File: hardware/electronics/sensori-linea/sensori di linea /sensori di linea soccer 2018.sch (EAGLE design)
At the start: 21 parts, among them T1 BP103, T2 BP103, T3 BP103, T4 BP103

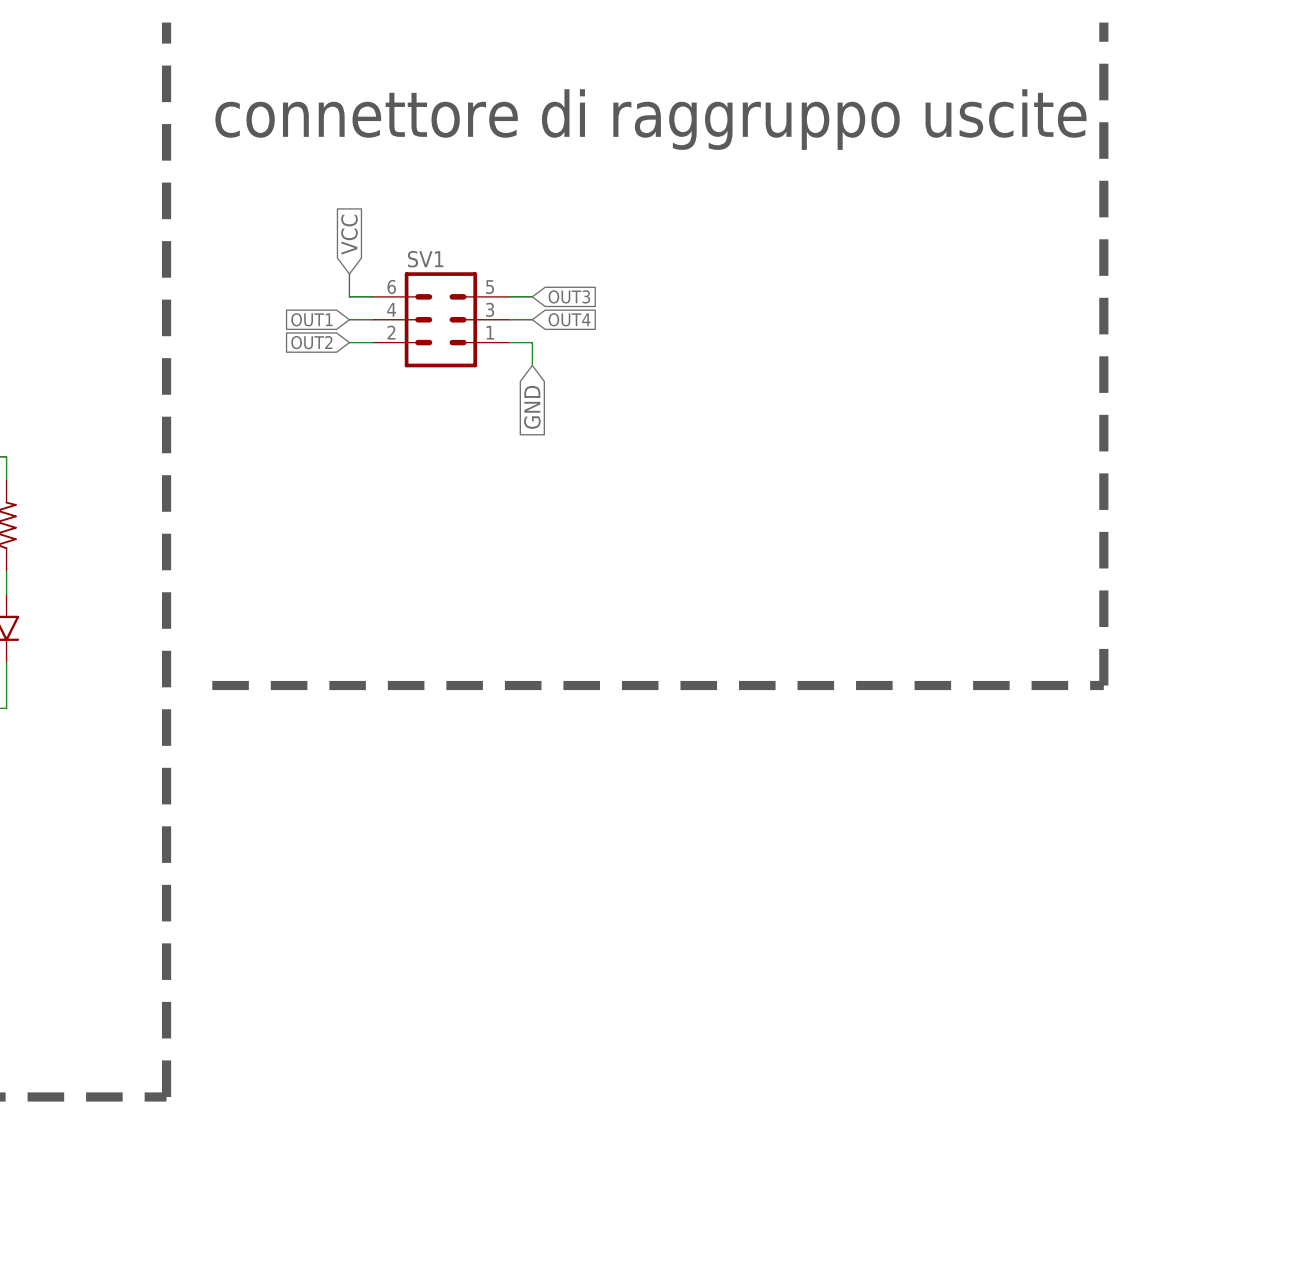
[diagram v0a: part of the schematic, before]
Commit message: aggiornamenti sensori
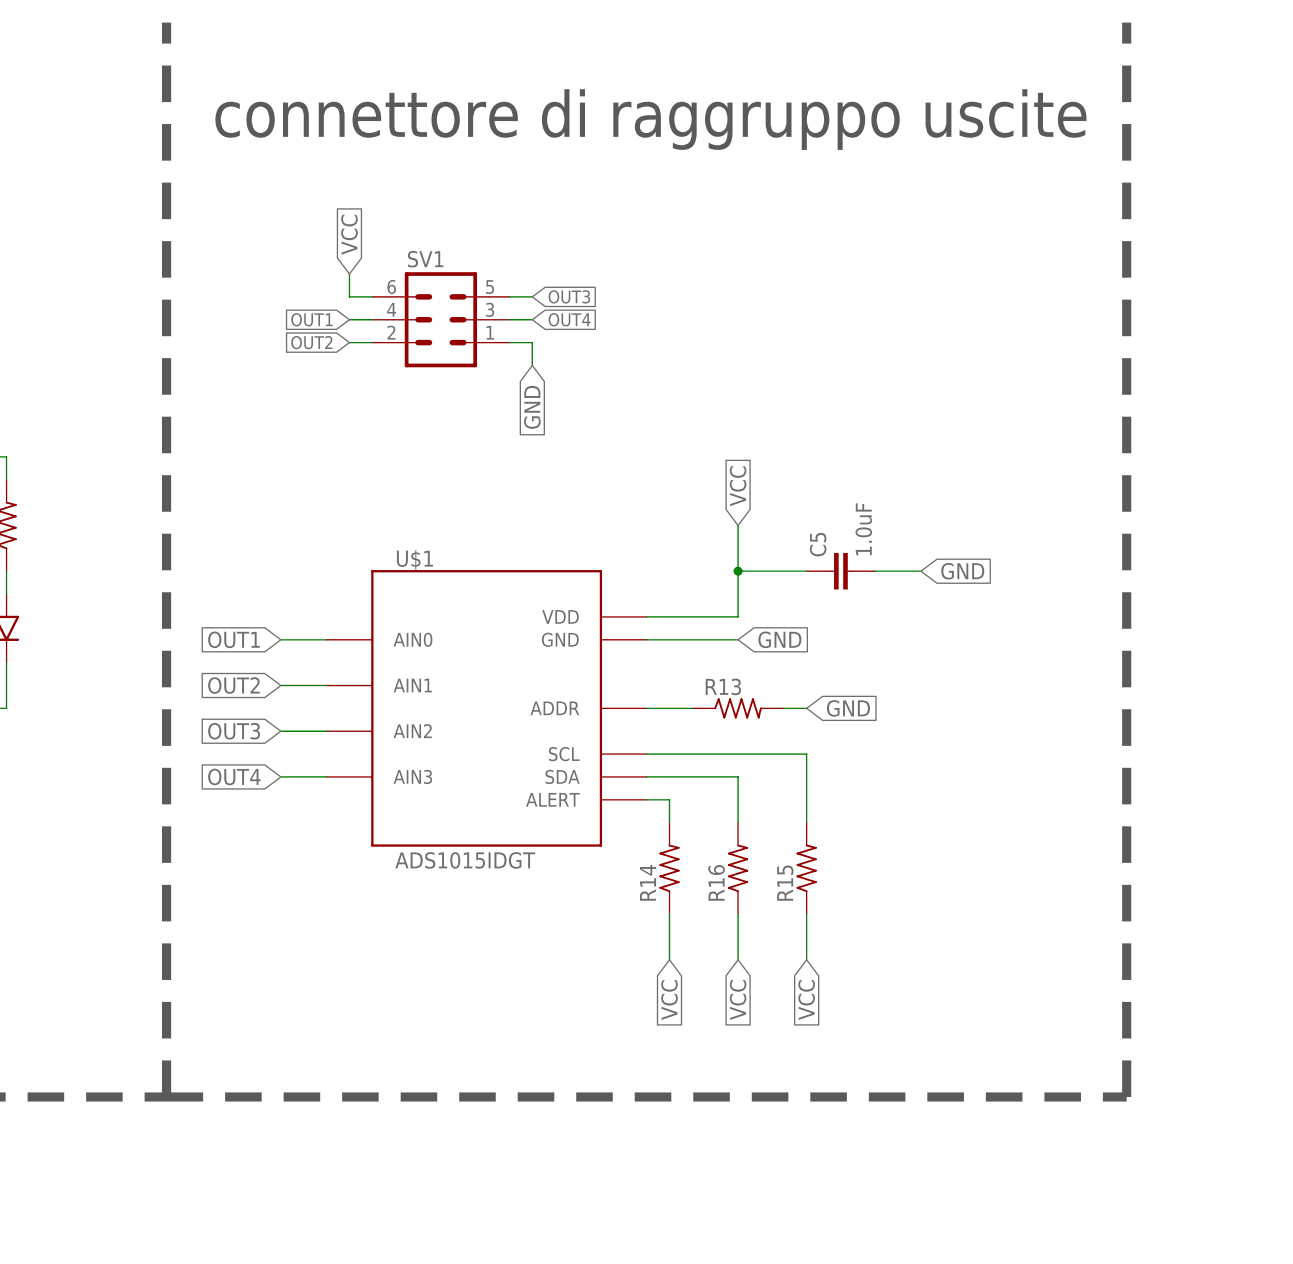
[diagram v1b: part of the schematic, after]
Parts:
- added C5: 1.0uF, SparkFun-Capacitors:1.0UF-0402-16V-10%
- added R13, R14, R15, R16: (no value), resistor:R-US_0204/7
- added U$1: ADS1015IDGT, bt_adc:ADS1015IDGT
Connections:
- new net N$1: R13.1, U$1.ADDR
- new net N$6: R16.2, U$1.SDA
- new net N$7: R14.2, U$1.ALERT
- new net N$8: R15.2, U$1.SCL
- net GND: now also C5.2, R13.2, U$1.GND
- net OUT1: now also U$1.AIN0
- net OUT2: now also U$1.AIN1
- net OUT3: now also U$1.AIN2
- net OUT4: now also U$1.AIN3
- net VCC: now also C5.1, R14.1, R15.1, R16.1, U$1.VDD
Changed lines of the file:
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@@
 <layers>
 <layer number="1" name="Top" color="4" fill="1" visible="no" active="no"/>
+<layer number="2" name="Route2" color="1" fill="3" visible="no" active="no"/>
+<layer number="3" name="Route3" color="4" fill="3" visible="no" active="no"/>
+<layer number="4" name="Route4" color="1" fill="4" visible="no" active="no"/>
+<layer number="5" name="Route5" color="4" fill="4" visible="no" active="no"/>
+<layer number="6" name="Route6" color="1" fill="8" visible="no" active="no"/>
+<layer number="7" name="Route7" color="4" fill="8" visible="no" active="no"/>
+<layer number="8" name="Route8" color="1" fill="2" visible="no" active="no"/>
+<layer number="9" name="Route9" color="4" fill="2" visible="no" active="no"/>
+<layer number="10" name="Route10" color="1" fill="7" visible="no" active="no"/>
+<layer number="11" name="Route11" color="4" fill="7" visible="no" active="no"/>
+<layer number="12" name="Route12" color="1" fill="5" visible="no" active="no"/>
+<layer number="13" name="Route13" color="4" fill="5" visible="no" active="no"/>
+<layer number="14" name="Route14" color="1" fill="6" visible="no" active="no"/>
+<layer number="15" name="Route15" color="4" fill="6" visible="no" active="no"/>
 <layer number="16" name="Bottom" color="1" fill="1" visible="no" active="no"/>
 <layer number="17" name="Pads" color="2" fill="1" visible="no" active="no"/>
@@
 <part name="D7" library="SparkFun-LED" deviceset="LED" device="3MM"/>
 <part name="D8" library="SparkFun-LED" deviceset="LED" device="3MM"/>
+<part name="U$1" library="bt_adc" deviceset="ADS1015" device="IDGT"/>
+<part name="C5" library="SparkFun-Capacitors" deviceset="1.0UF" device="-0402-16V-10%" value="1.0uF"/>
+<part name="R13" library="resistor" library_urn="urn:adsk.eagle:library:348" deviceset="R-US_" device="0204/7" package3d_urn="urn:adsk.eagle:package:25945/1"/>
+<part name="R14" library="resistor" library_urn="urn:adsk.eagle:library:348" deviceset="R-US_" device="0204/7" package3d_urn="urn:adsk.eagle:package:25945/1"/>
+<part name="R15" library="resistor" library_urn="urn:adsk.eagle:library:348" deviceset="R-US_" device="0204/7" package3d_urn="urn:adsk.eagle:package:25945/1"/>
+<part name="R16" library="resistor" library_urn="urn:adsk.eagle:library:348" deviceset="R-US_" device="0204/7" package3d_urn="urn:adsk.eagle:package:25945/1"/>
 </parts>
 <sheets>
@@
 <wire x1="165.1" y1="132.08" x2="226.06" y2="132.08" width="1.016" layer="97" style="longdash"/>
 <wire x1="226.06" y1="132.08" x2="226.06" y2="251.46" width="1.016" layer="97" style="longdash"/>
-<wire x1="231.14" y1="177.8" x2="330.2" y2="177.8" width="1.016" layer="97" style="longdash"/>
-<wire x1="330.2" y1="177.8" x2="330.2" y2="251.46" width="1.016" layer="97" style="longdash"/>
 <text x="325.12" y="7.62" size="1.778" layer="95">progettato e realizzato da Francesco Spena</text>
+<wire x1="226.06" y1="132.08" x2="332.74" y2="132.08" width="1.016" layer="97" style="longdash"/>
+<wire x1="332.74" y1="132.08" x2="332.74" y2="251.46" width="1.016" layer="97" style="longdash"/>
 </plain>
 <instances>
@@
 <instance part="D7" gate="G$1" x="198.12" y="185.42"/>
 <instance part="D8" gate="G$1" x="208.28" y="185.42"/>
+<instance part="U$1" gate="G$1" x="261.62" y="175.26"/>
+<instance part="C5" gate="G$1" x="302.26" y="190.5" rot="R90"/>
+<instance part="R13" gate="G$1" x="289.56" y="175.26"/>
+<instance part="R14" gate="G$1" x="281.94" y="157.48" rot="R90"/>
+<instance part="R15" gate="G$1" x="297.18" y="157.48" rot="R90"/>
+<instance part="R16" gate="G$1" x="289.56" y="157.48" rot="R90"/>
 </instances>
 <busses>
@@
 <label x="246.38" y="223.52" size="1.778" layer="95" rot="R90" xref="yes"/>
 </segment>
+<segment>
+<pinref part="U$1" gate="G$1" pin="VDD"/>
+<wire x1="279.4" y1="185.42" x2="289.56" y2="185.42" width="0.1524" layer="91"/>
+<label x="289.56" y="195.58" size="1.778" layer="95" rot="R90" xref="yes"/>
+<pinref part="C5" gate="G$1" pin="1"/>
+<wire x1="289.56" y1="185.42" x2="289.56" y2="190.5" width="0.1524" layer="91"/>
+<wire x1="289.56" y1="190.5" x2="289.56" y2="195.58" width="0.1524" layer="91"/>
+<wire x1="297.18" y1="190.5" x2="289.56" y2="190.5" width="0.1524" layer="91"/>
+<junction x="289.56" y="190.5"/>
+</segment>
+<segment>
+<wire x1="281.94" y1="152.4" x2="281.94" y2="147.32" width="0.1524" layer="91"/>
+<label x="281.94" y="147.32" size="1.778" layer="95" rot="R270" xref="yes"/>
+<pinref part="R14" gate="G$1" pin="1"/>
+</segment>
+<segment>
+<wire x1="289.56" y1="152.4" x2="289.56" y2="147.32" width="0.1524" layer="91"/>
+<label x="289.56" y="147.32" size="1.778" layer="95" rot="R270" xref="yes"/>
+<pinref part="R16" gate="G$1" pin="1"/>
+</segment>
+<segment>
+<wire x1="297.18" y1="152.4" x2="297.18" y2="147.32" width="0.1524" layer="91"/>
+<label x="297.18" y="147.32" size="1.778" layer="95" rot="R270" xref="yes"/>
+<pinref part="R15" gate="G$1" pin="1"/>
+</segment>
 </net>
 <net name="OUT1" class="0">
@@
 <wire x1="248.92" y1="218.44" x2="246.38" y2="218.44" width="0.1524" layer="91"/>
 <label x="246.38" y="218.44" size="1.4224" layer="95" rot="R180" xref="yes"/>
+</segment>
+<segment>
+<pinref part="U$1" gate="G$1" pin="AIN0"/>
+<wire x1="243.84" y1="182.88" x2="238.76" y2="182.88" width="0.1524" layer="91"/>
+<label x="238.76" y="182.88" size="1.778" layer="95" rot="R180" xref="yes"/>
 </segment>
 </net>
@@
 <label x="134.62" y="149.86" size="1.4224" layer="95" rot="R270" xref="yes"/>
 </segment>
+<segment>
+<pinref part="U$1" gate="G$1" pin="GND"/>
+<wire x1="279.4" y1="182.88" x2="289.56" y2="182.88" width="0.1524" layer="91"/>
+<label x="289.56" y="182.88" size="1.778" layer="95" xref="yes"/>
+</segment>
+<segment>
+<wire x1="294.64" y1="175.26" x2="297.18" y2="175.26" width="0.1524" layer="91"/>
+<label x="297.18" y="175.26" size="1.778" layer="95" xref="yes"/>
+<pinref part="R13" gate="G$1" pin="2"/>
+</segment>
+<segment>
+<pinref part="C5" gate="G$1" pin="2"/>
+<wire x1="304.8" y1="190.5" x2="309.88" y2="190.5" width="0.1524" layer="91"/>
+<label x="309.88" y="190.5" size="1.778" layer="95" xref="yes"/>
+</segment>
 </net>
 <net name="OUT2" class="0">
@@
 <label x="246.38" y="215.9" size="1.4224" layer="95" rot="R180" xref="yes"/>
 </segment>
+<segment>
+<pinref part="U$1" gate="G$1" pin="AIN1"/>
+<wire x1="243.84" y1="177.8" x2="238.76" y2="177.8" width="0.1524" layer="91"/>
+<label x="238.76" y="177.8" size="1.778" layer="95" rot="R180" xref="yes"/>
+</segment>
 </net>
 <net name="OUT3" class="0">
@@
 <wire x1="264.16" y1="220.98" x2="266.7" y2="220.98" width="0.1524" layer="91"/>
 <label x="266.7" y="220.98" size="1.4224" layer="95" xref="yes"/>
+</segment>
+<segment>
+<pinref part="U$1" gate="G$1" pin="AIN2"/>
+<wire x1="243.84" y1="172.72" x2="238.76" y2="172.72" width="0.1524" layer="91"/>
+<label x="238.76" y="172.72" size="1.778" layer="95" rot="R180" xref="yes"/>
 </segment>
 </net>
@@
 <label x="266.7" y="218.44" size="1.4224" layer="95" xref="yes"/>
 </segment>
+<segment>
+<pinref part="U$1" gate="G$1" pin="AIN3"/>
+<wire x1="243.84" y1="167.64" x2="238.76" y2="167.64" width="0.1524" layer="91"/>
+<label x="238.76" y="167.64" size="1.778" layer="95" rot="R180" xref="yes"/>
+</segment>
 </net>
 <net name="N$2" class="0">
@@
 </segment>
 </net>
+<net name="N$1" class="0">
+<segment>
+<pinref part="U$1" gate="G$1" pin="ADDR"/>
+<wire x1="279.4" y1="175.26" x2="284.48" y2="175.26" width="0.1524" layer="91"/>
+<pinref part="R13" gate="G$1" pin="1"/>
+</segment>
+</net>
+<net name="N$7" class="0">
+<segment>
+<pinref part="U$1" gate="G$1" pin="ALERT"/>
+<wire x1="279.4" y1="165.1" x2="281.94" y2="165.1" width="0.1524" layer="91"/>
+<wire x1="281.94" y1="162.56" x2="281.94" y2="165.1" width="0.1524" layer="91"/>
+<pinref part="R14" gate="G$1" pin="2"/>
+</segment>
+</net>
+<net name="N$6" class="0">
+<segment>
+<pinref part="U$1" gate="G$1" pin="SDA"/>
+<wire x1="279.4" y1="167.64" x2="289.56" y2="167.64" width="0.1524" layer="91"/>
+<wire x1="289.56" y1="167.64" x2="289.56" y2="162.56" width="0.1524" layer="91"/>
+<pinref part="R16" gate="G$1" pin="2"/>
+</segment>
+</net>
+<net name="N$8" class="0">
+<segment>
+<pinref part="U$1" gate="G$1" pin="SCL"/>
+<wire x1="279.4" y1="170.18" x2="297.18" y2="170.18" width="0.1524" layer="91"/>
+<wire x1="297.18" y1="170.18" x2="297.18" y2="162.56" width="0.1524" layer="91"/>
+<pinref part="R15" gate="G$1" pin="2"/>
+</segment>
+</net>
